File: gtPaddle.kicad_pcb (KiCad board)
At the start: 2 copper layers, 51.4 x 72.6 mm, 44 parts, among them IC1 74157N, IC2 74157N, J1 Conn_01x02_Pin, J2 Conn_01x02_Pin, J3 Conn_01x02_Pin, J4 Conn_01x02_Pin, Q1 2N3904, Q10 2N3904, Q2 2N3904, Q3 2N3904, Q9 2N3904, U1 ADC0804LCN

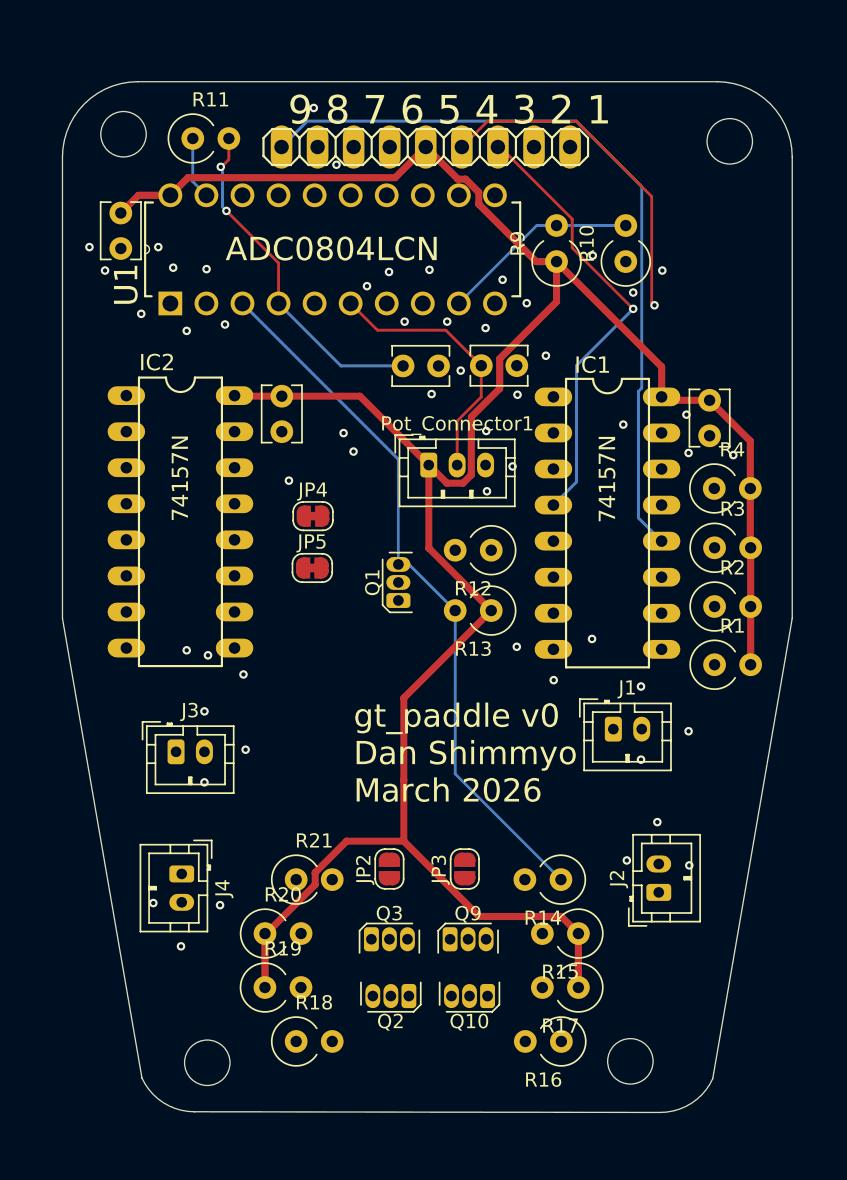
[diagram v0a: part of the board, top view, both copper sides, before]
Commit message: remove npn muxes
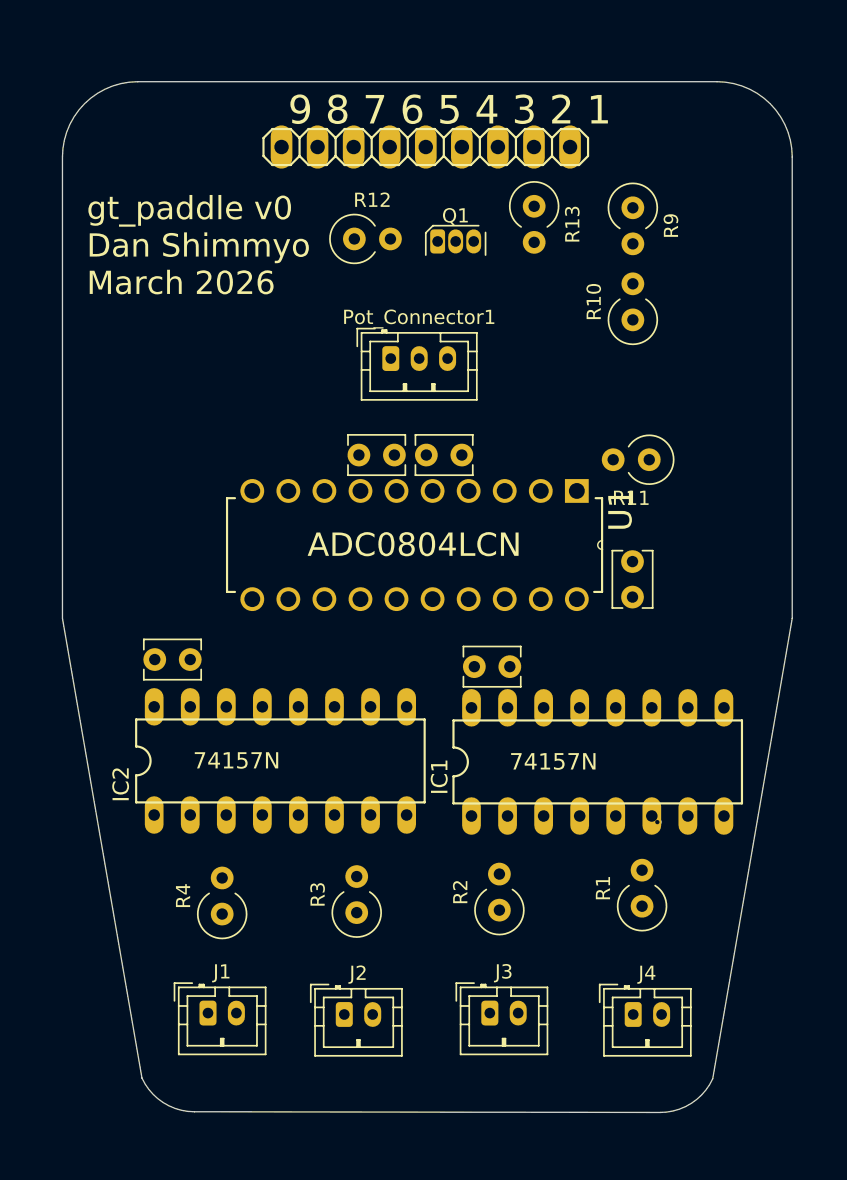
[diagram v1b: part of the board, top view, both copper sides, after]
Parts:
- removed ? (x4): , 
- removed JP2, JP3: SolderJumper_2_Open, Jumper:SolderJumper-2_P1.3mm_Open_RoundedPad1.0x1.5mm
- removed JP4, JP5: SolderJumper_2_Bridged, Jumper:SolderJumper-2_P1.3mm_Bridged_RoundedPad1.0x1.5mm
- removed Q10, Q2, Q3, Q9: 2N3904, Package_TO_SOT_THT:TO-92S-EBC
- removed R14, R16, R18, R21: 10K, Resistor_THT:R_Axial_DIN0309_L9.0mm_D3.2mm_P2.54mm_Vertical
- removed R15, R17, R19, R20: 3.3K, Resistor_THT:R_Axial_DIN0309_L9.0mm_D3.2mm_P2.54mm_Vertical
- moved R4 45.8 mm to (136.7, 126.2), turned to 90 degrees
- moved C5 45.1 mm to (165.6, 103.9), turned to 90 degrees
- moved R11 39.3 mm to (166.7, 94.2), turned to 180 degrees
- moved R3 36.0 mm to (146.1, 126.1), turned to 90 degrees
- moved J1 34.9 mm to (135.7, 133.2)
- moved J4 33.3 mm to (165.6, 133.3), turned to 0 degrees
- moved U1 33.2 mm to (138.8, 104.0), turned to -90 degrees
- moved J3 28.8 mm to (155.5, 133.2)
- moved R13 28.6 mm to (158.6, 76.4), turned to -90 degrees
- moved R2 26.2 mm to (156.2, 126.0), turned to 90 degrees
- moved Q1 25.4 mm to (151.8, 78.8), turned to 0 degrees
- moved C4 25.0 mm to (154.4, 108.8), turned to 0 degrees
- moved R12 24.0 mm to (146.0, 78.7), turned to 0 degrees
- moved J2 23.8 mm to (145.2, 133.3), turned to 0 degrees
- moved C3 20.6 mm to (131.9, 108.3), turned to 0 degrees
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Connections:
- JP1 pad 1: Net-(JP2-B) -> Net-(IC2A-1Y)
- JP1 pad 2: Net-(JP3-B) -> Net-(IC2A-2Y)
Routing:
- net VCC: track 175.8 -> 0.00 mm
- net Net-(IC1A-4Y): track 53.8 -> 0.00 mm
- net Net-(Q1-C): track 50.3 -> 0.00 mm
- net Net-(IC1A-1Y): track 31.6 -> 0.00 mm, vias 1 -> 0
- net Net-(U1-CLK_IN): track 24.3 -> 0.00 mm, vias 2 -> 0
- net Net-(IC1A-2Y): track 24.1 -> 0.00 mm, vias 1 -> 0
- net Net-(Pot_Connector1-Pin_2): track 18.7 -> 0.00 mm
- net Net-(U1-VREF/2): track 14.0 -> 0.00 mm
- net Net-(U1-CLK_R): track 4.40 -> 0.00 mm
- net GND: vias 53 -> 1

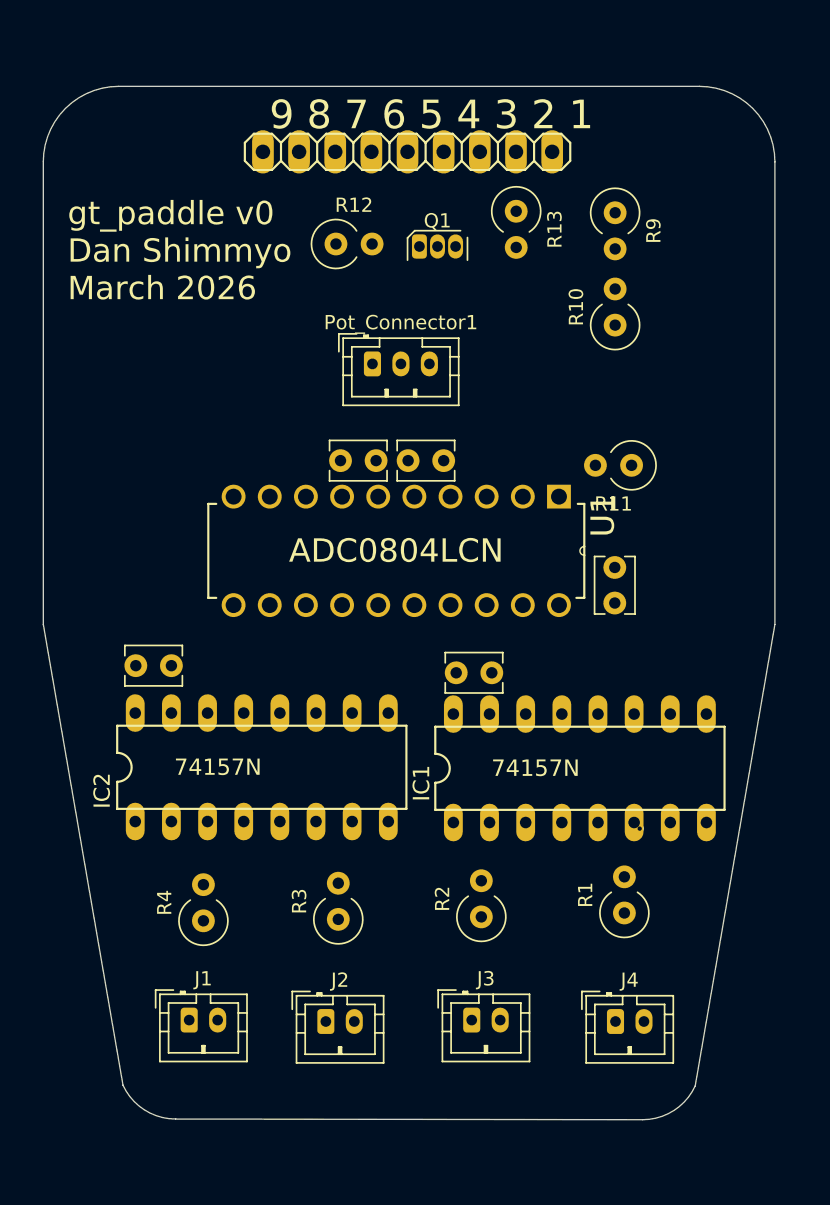
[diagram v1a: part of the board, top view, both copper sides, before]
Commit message: layout tweaks
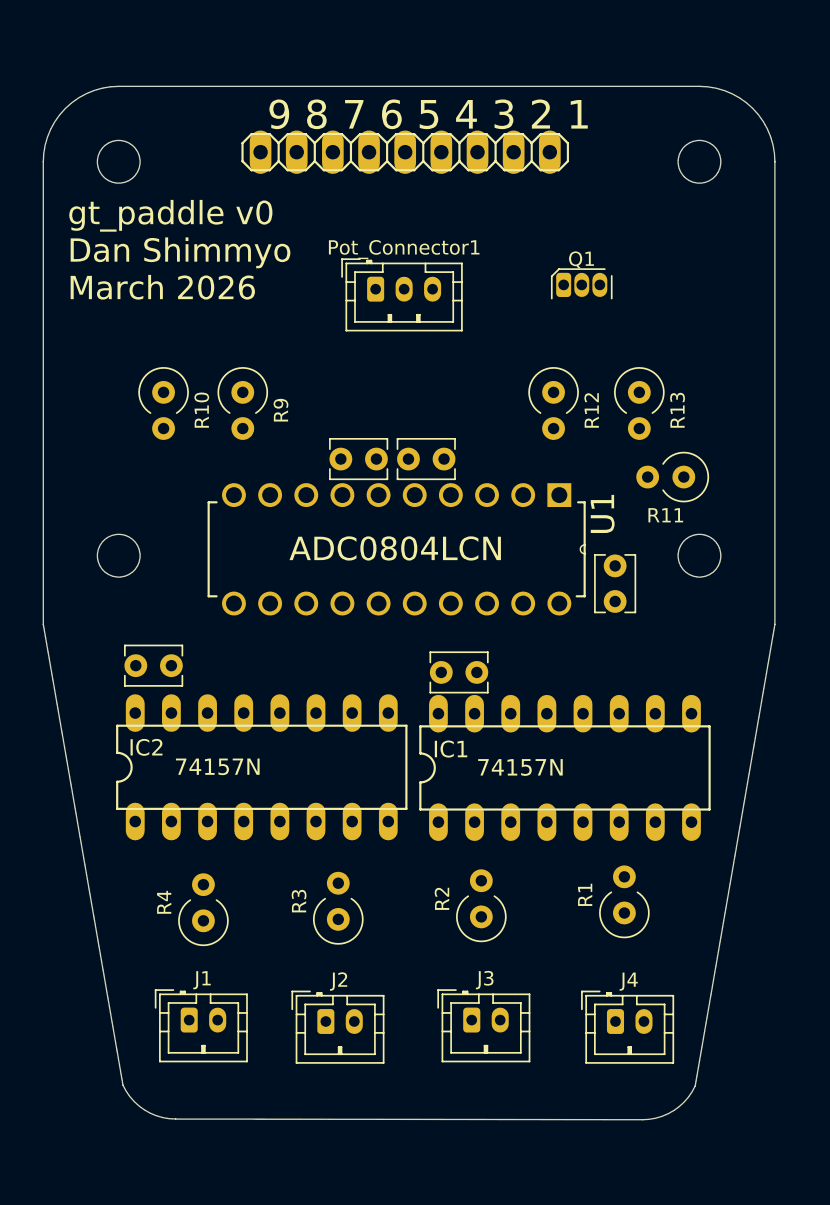
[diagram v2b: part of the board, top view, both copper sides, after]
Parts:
- added ?: , , F.Cu at (130.7, 72.9)
- added ?: , , F.Cu at (171.5, 72.9)
- added ?: , , F.Cu at (171.5, 100.6)
- added ?: , , F.Cu at (130.7, 100.6)
- moved R10 32.1 mm to (133.8, 89.1), turned to -90 degrees
- moved R9 29.0 mm to (139.4, 89.1)
- moved R12 18.5 mm to (161.2, 89.1), turned to -90 degrees
- moved R13 15.4 mm to (167.3, 89.1)
- moved Q1 10.5 mm to (162.0, 81.5)
- moved Pot_Connector1 5.25 mm to (148.8, 81.8)
- moved R11 3.76 mm to (170.4, 95.0)
- moved IC1 1.05 mm to (162.1, 115.5)
- moved C4 1.05 mm to (153.4, 108.8)
- moved JP1 0.17 mm to (150.8, 72.2)
- moved C1 0.11 mm to (153.6, 93.8)
- moved C2 0.11 mm to (146.3, 93.8)
- moved C5 0.11 mm to (165.6, 103.8)
- moved U1 0.11 mm to (138.8, 103.9)
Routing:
- net GND: vias 1 -> 0
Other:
- board text added: "1 2 3 4 5 6 7 8 9"
